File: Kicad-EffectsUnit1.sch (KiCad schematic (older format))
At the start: 110 parts, among them J101 In7, J102 Doepfer connector, J103 Vin 7-12v, J104 In6, J105 In3, J106 Out10, J107 Out11, J108 Out12, J109 Out13, J110 Power Conn, SW101 SW_DPDT_x2, SW102 SW_SPDT, SW103 Rotary_Encoder_Switch, U101 TL072, U102 TL072

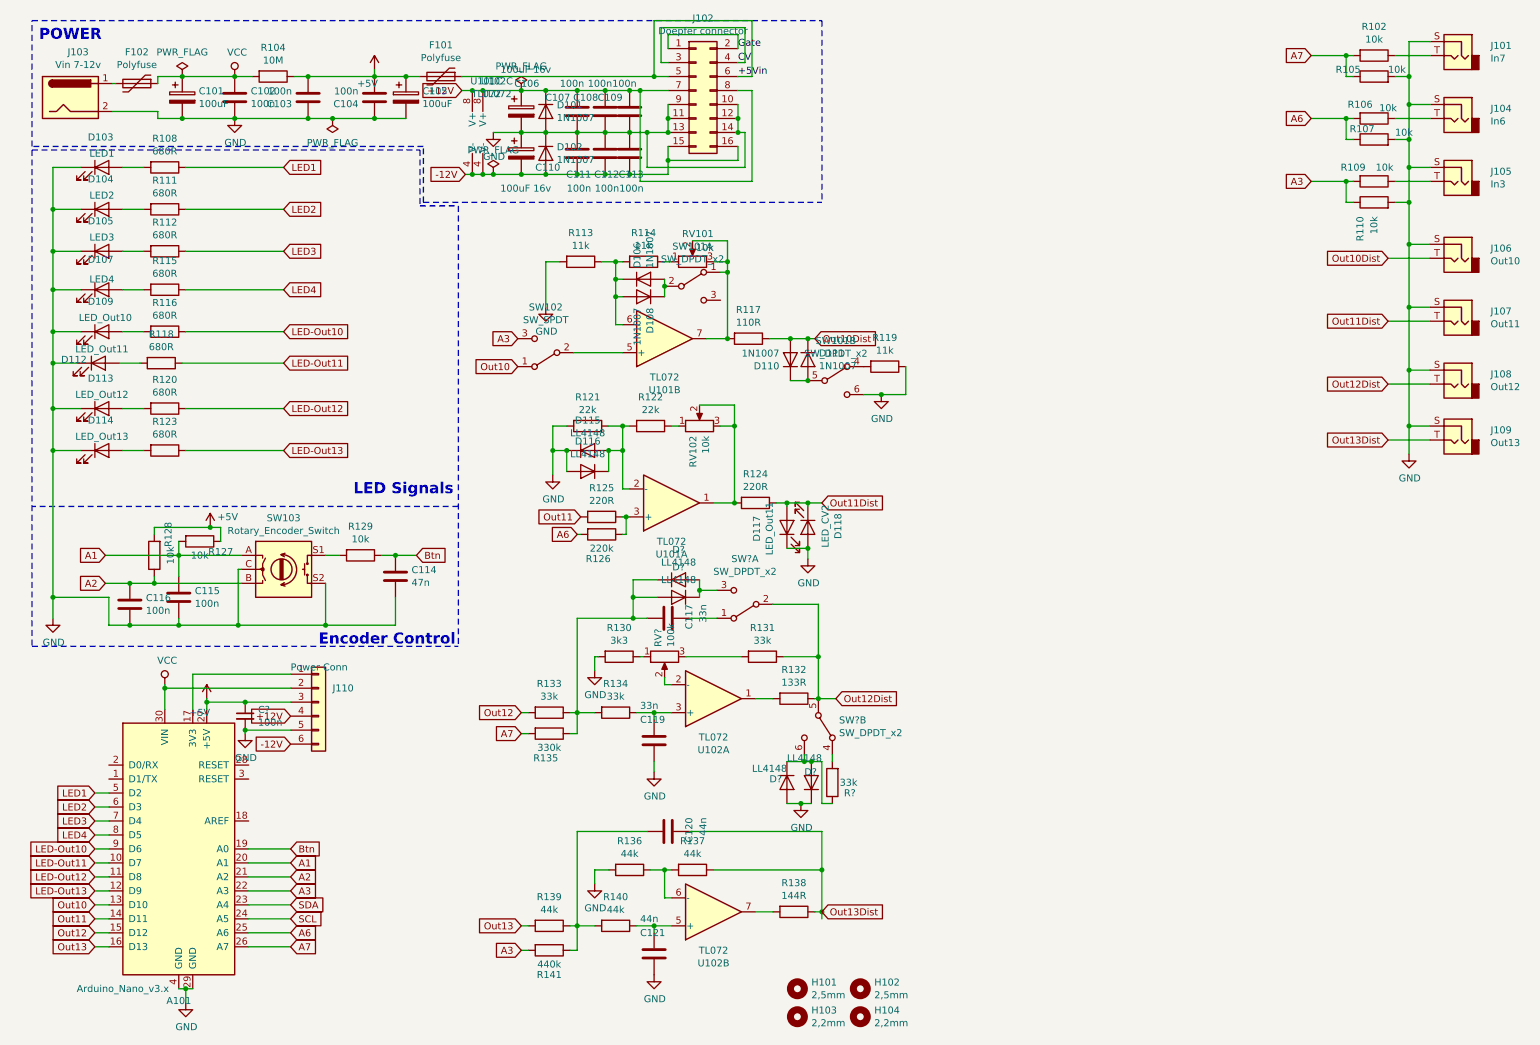
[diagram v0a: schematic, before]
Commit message: PT2399 started
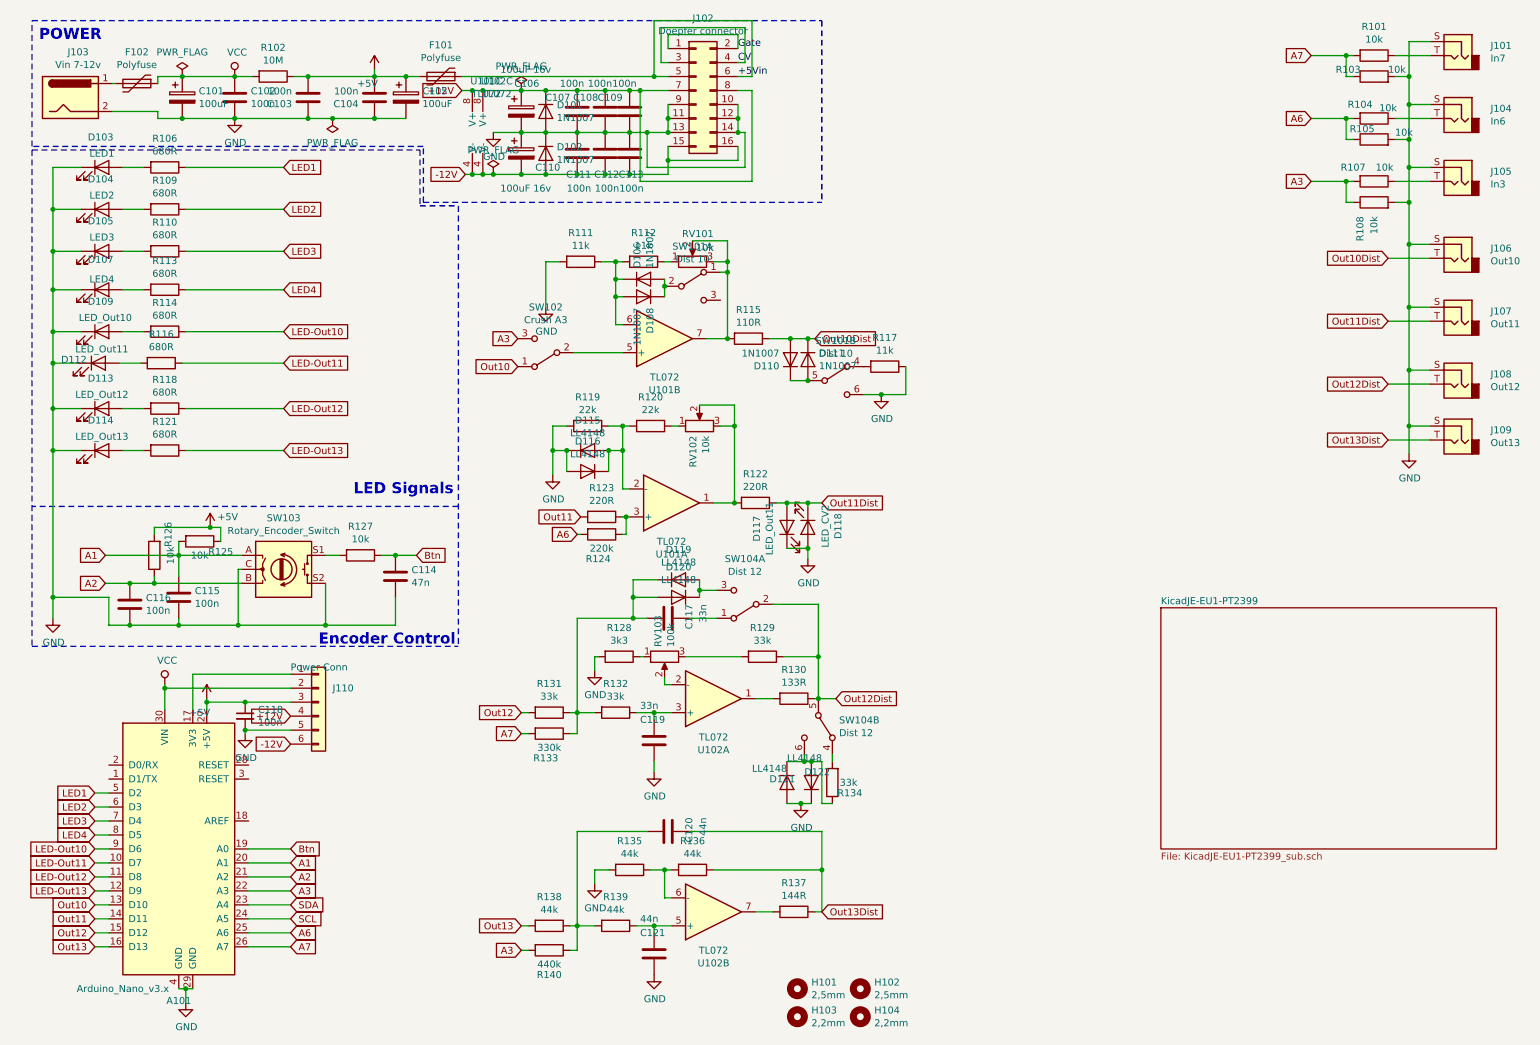
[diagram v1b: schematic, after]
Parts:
- SW101: value SW_DPDT_x2 -> Dist 10
- SW102: value SW_SPDT -> Crush A3
- SW104: renamed from SW?; value SW_DPDT_x2 -> Dist 12
- gave numbers to parts that had none: 7
- renumbered R102 to R101, R104 to R102, R105 to R103, R106 to R104, R107 to R105, R108 to R106, R109 to R107, R110 to R108, R111 to R109, R112 to R110, R113 to R111, R114 to R112, R115 to R113, R116 to R114, R117 to R115, R118 to R116, R119 to R117, R120 to R118, R121 to R119, R122 to R120, R123 to R121, R124 to R122, R125 to R123, R126 to R124, R127 to R125, R128 to R126, R129 to R127, R130 to R128, R131 to R129, R132 to R130, R133 to R131, R134 to R132, R135 to R133, R136 to R135, R137 to R136, R138 to R137, R139 to R138, R140 to R139, R141 to R140

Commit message: more footprints
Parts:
- J101, J104, J105, J108, J109: footprint Connector_Audio:AudioJack3StereoNarrow-PJ-321 -> AJ-Dropbox-Kicad:PJ301SM
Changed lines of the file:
@@
 F 0 "J108" H 10567 3171 50  0000 R CNN
 F 1 "Out12" H 10567 3080 50  0000 R CNN
-F 2 "Connector_Audio:AudioJack3StereoNarrow-PJ-321" H 10800 3100 50  0001 C CNN
+F 2 "AJ-Dropbox-Kicad:PJ301SM" H 10800 3100 50  0001 C CNN
 F 3 "~" H 10800 3100 50  0001 C CNN
 	1    10800 3100
@@
 F 0 "J109" H 10567 3571 50  0000 R CNN
 F 1 "Out13" H 10567 3480 50  0000 R CNN
-F 2 "Connector_Audio:AudioJack3StereoNarrow-PJ-321" H 10800 3500 50  0001 C CNN
+F 2 "AJ-Dropbox-Kicad:PJ301SM" H 10800 3500 50  0001 C CNN
 F 3 "~" H 10800 3500 50  0001 C CNN
 	1    10800 3500
@@
 F 0 "J104" H 10567 1271 50  0000 R CNN
 F 1 "In6" H 10567 1180 50  0000 R CNN
-F 2 "Connector_Audio:AudioJack3StereoNarrow-PJ-321" H 10800 1200 50  0001 C CNN
+F 2 "AJ-Dropbox-Kicad:PJ301SM" H 10800 1200 50  0001 C CNN
 F 3 "~" H 10800 1200 50  0001 C CNN
 F 4 "VC input" H 10800 1200 50  0001 C CNN "Function"
@@
 F 0 "J101" H 10567 821 50  0000 R CNN
 F 1 "In7" H 10567 730 50  0000 R CNN
-F 2 "Connector_Audio:AudioJack3StereoNarrow-PJ-321" H 10800 750 50  0001 C CNN
+F 2 "AJ-Dropbox-Kicad:PJ301SM" H 10800 750 50  0001 C CNN
 F 3 "~" H 10800 750 50  0001 C CNN
 F 4 "VC input" H 10800 750 50  0001 C CNN "Function"
@@
 F 0 "J105" H 10567 1721 50  0000 R CNN
 F 1 "In3" H 10567 1630 50  0000 R CNN
-F 2 "Connector_Audio:AudioJack3StereoNarrow-PJ-321" H 10800 1650 50  0001 C CNN
+F 2 "AJ-Dropbox-Kicad:PJ301SM" H 10800 1650 50  0001 C CNN
 F 3 "~" H 10800 1650 50  0001 C CNN
 F 4 "VC input" H 10800 1650 50  0001 C CNN "Function"
